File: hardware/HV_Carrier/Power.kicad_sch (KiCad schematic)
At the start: 12 parts, among them J8 USB_C_Receptacle_USB2.0_16P

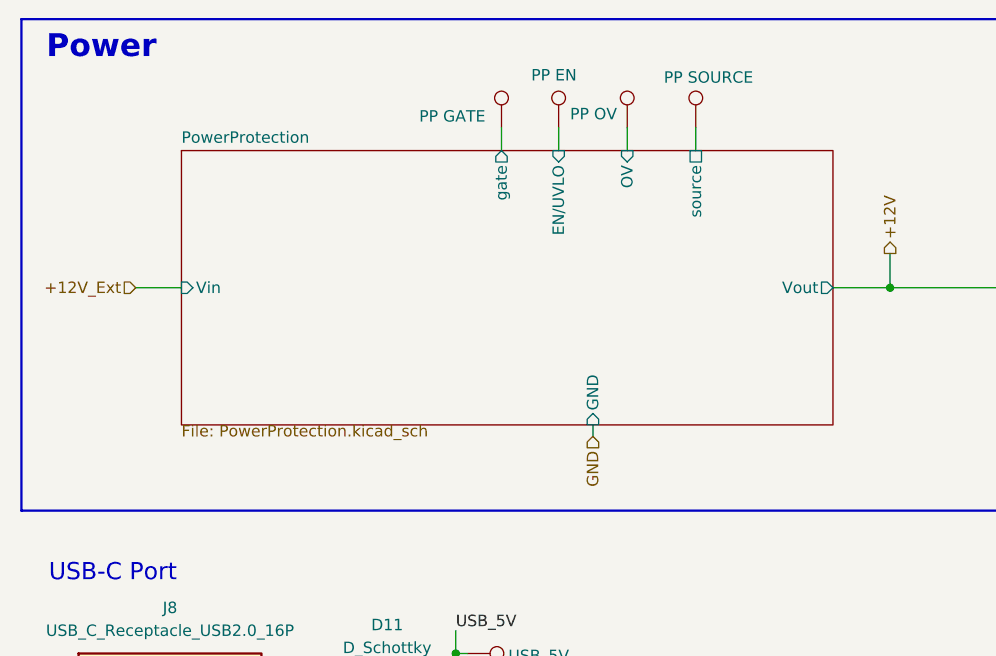
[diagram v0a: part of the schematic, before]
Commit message: updatred PP
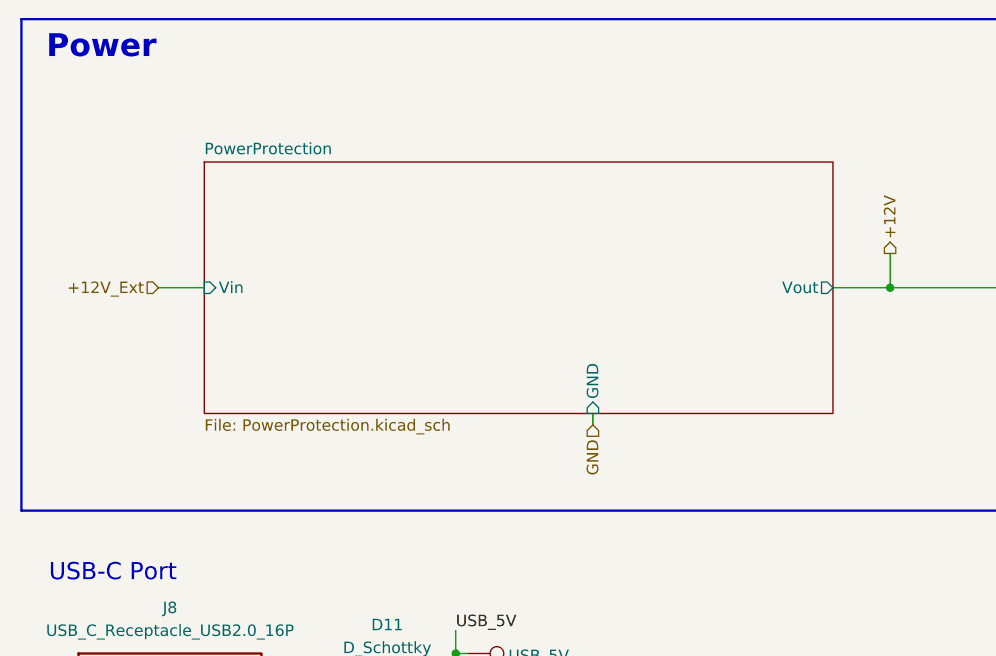
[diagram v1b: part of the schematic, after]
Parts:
- removed TP10: PP OV, TestPoint:TestPoint_THTPad_D3.0mm_Drill1.5mm, symbol Connector:TestPoint
- removed TP11: PP SOURCE, TestPoint:TestPoint_THTPad_D3.0mm_Drill1.5mm, symbol Connector:TestPoint
- removed TP8: PP GATE, TestPoint:TestPoint_THTPad_D3.0mm_Drill1.5mm, symbol Connector:TestPoint
- removed TP9: PP EN, TestPoint:TestPoint_THTPad_D3.0mm_Drill1.5mm, symbol Connector:TestPoint
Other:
- sheet PowerProtection ports: added none; removed EN/UVLO, OV, gate, source
